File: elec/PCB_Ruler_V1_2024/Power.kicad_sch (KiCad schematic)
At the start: 9 parts, among them U1 MCP73831T-2ACI_OT, U3 TLV75533PDBV

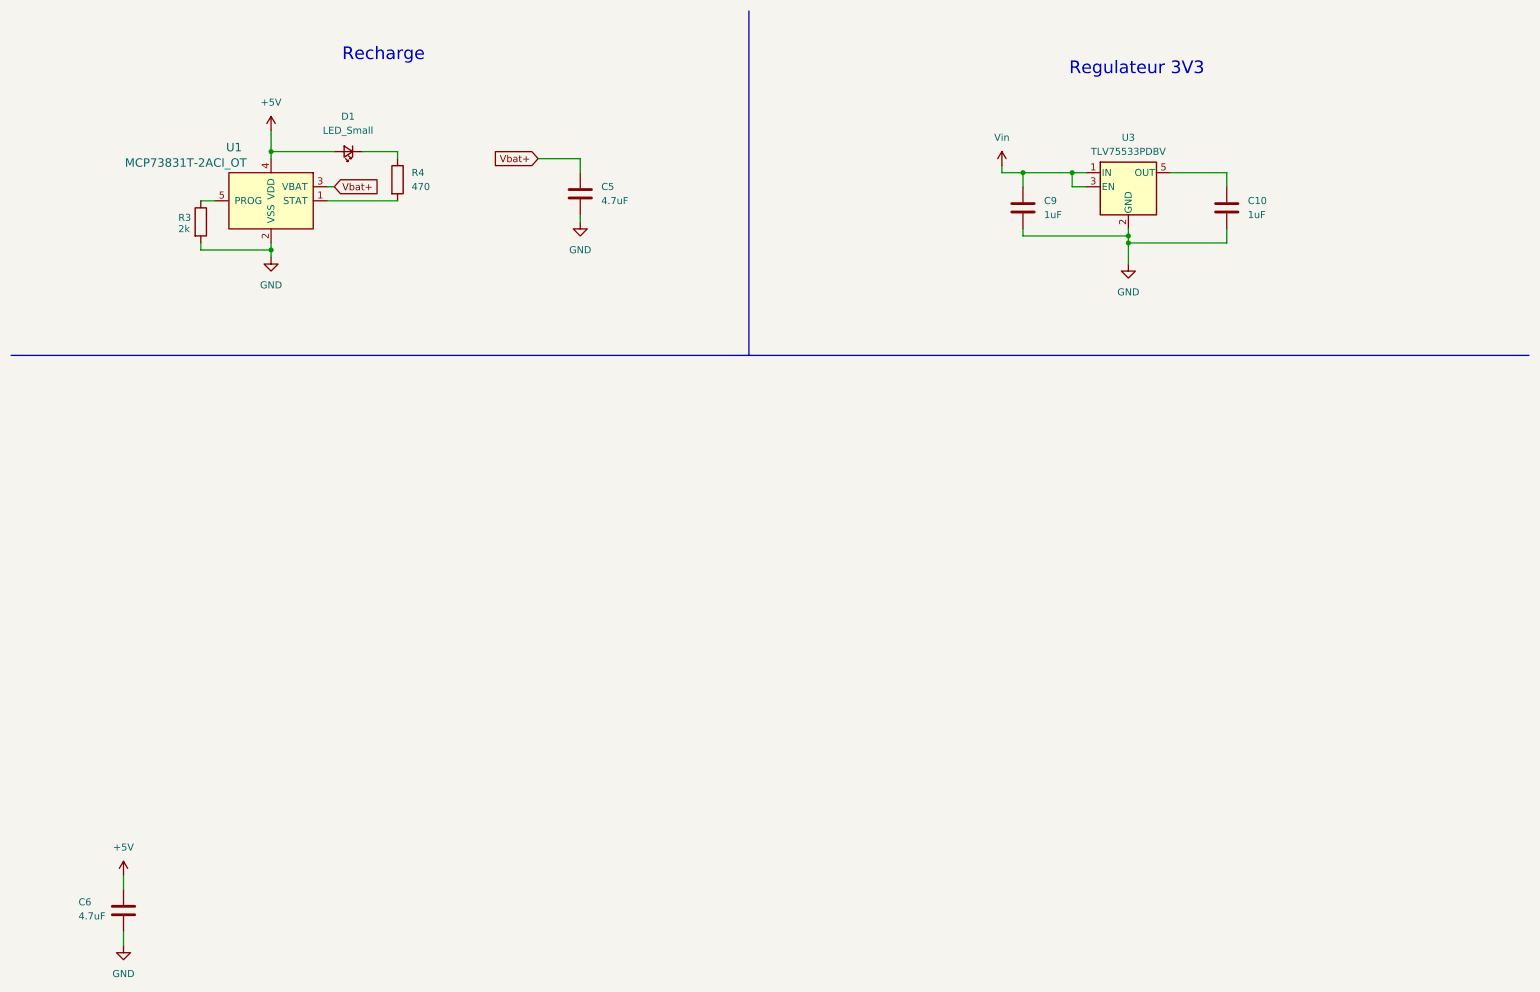
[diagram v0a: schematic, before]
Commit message: Almost finished schematic...
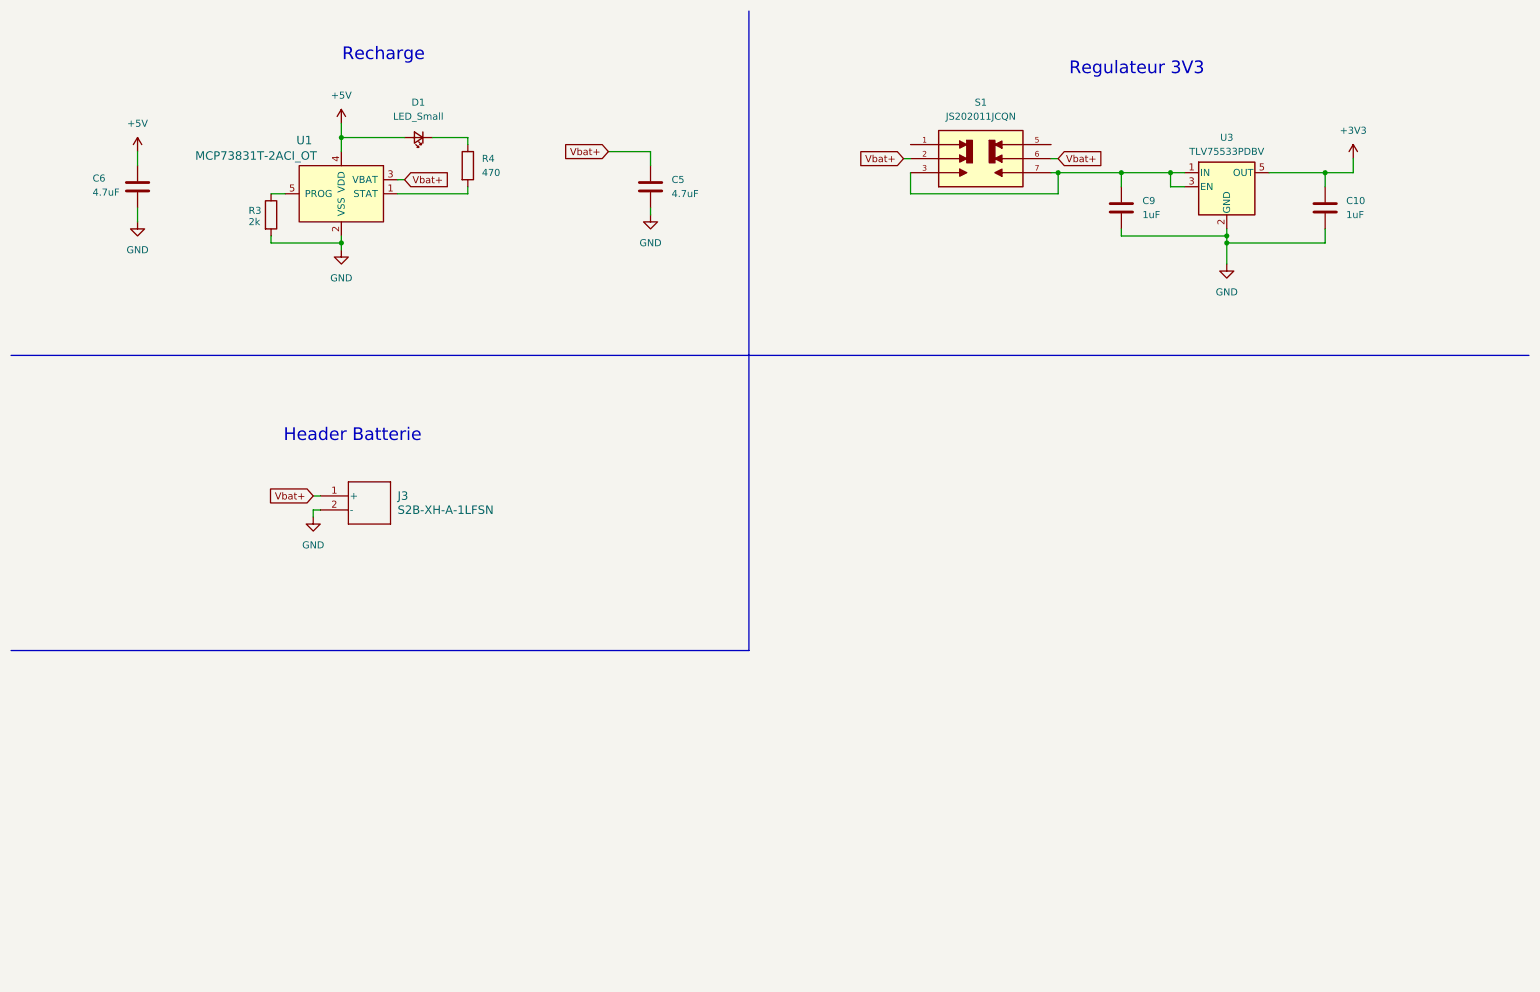
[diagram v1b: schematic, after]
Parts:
- added J3: S2B-XH-A-1LFSN, Connector_JST:JST_XH_S2B-XH-A-1_1x02_P2.50mm_Horizontal, symbol S2B-XH-A-1:S2B-XH-A-1LFSN
- added S1: JS202011JCQN, JS202011JCQN:SW_JS202011JCQN, symbol JS202011JCQN:JS202011JCQN
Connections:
- net GND: now also J3.2 (-)
- net Vbat+: now also J3.1 (+), S1.2, S1.6
- net +3V3: now reaches C10.1, U3.5 (OUT)
- net Vin: no longer names the net of C9.1, U3.1 (IN), U3.3 (EN)
- net Vin: now also S1.3, S1.7
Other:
- note added: "Header Batterie"
- moved on the sheet: C10, C5, C6, C9, D1, R3, R4, U1, U3
